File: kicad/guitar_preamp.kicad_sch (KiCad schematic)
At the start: 42 parts, among them J1 IN (от SW1B, экранир. провод), J2 BAT+ (TP4056 OUT+), J3 OUT (к SW1A) / GND, J4 Выход 6.3 Mono, J5 Звукосниматели: COM/GND, J6 TP4056 OUT+/OUT-, J7 LED (A / K), SW1 DPDT push-pull RV1, U1 MCP6022/OPA2316

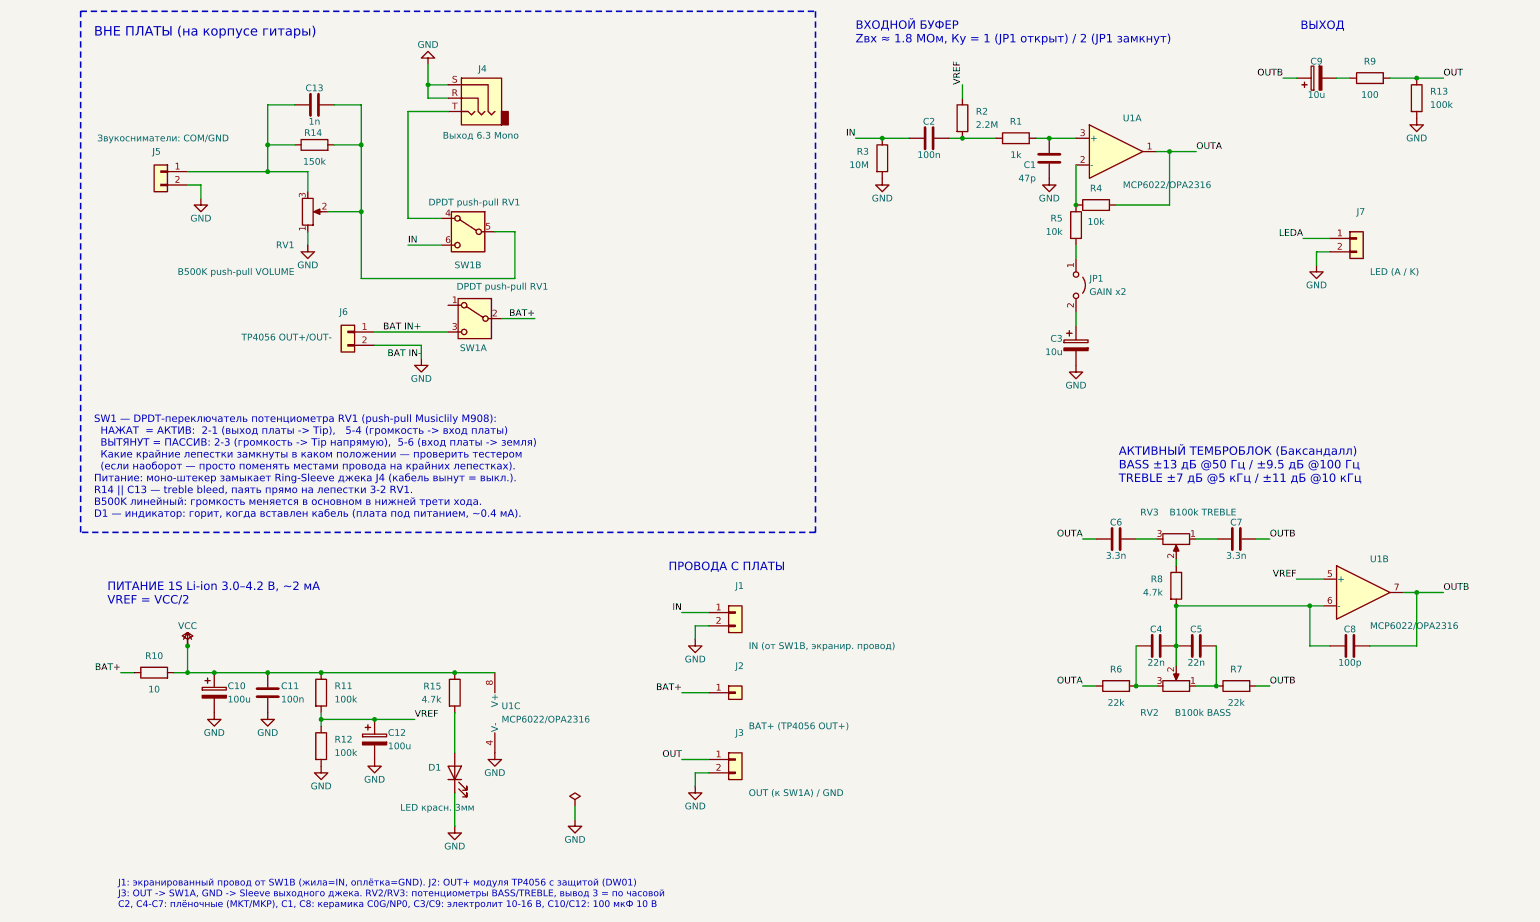
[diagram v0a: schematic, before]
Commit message: кутерьма с коннекторами
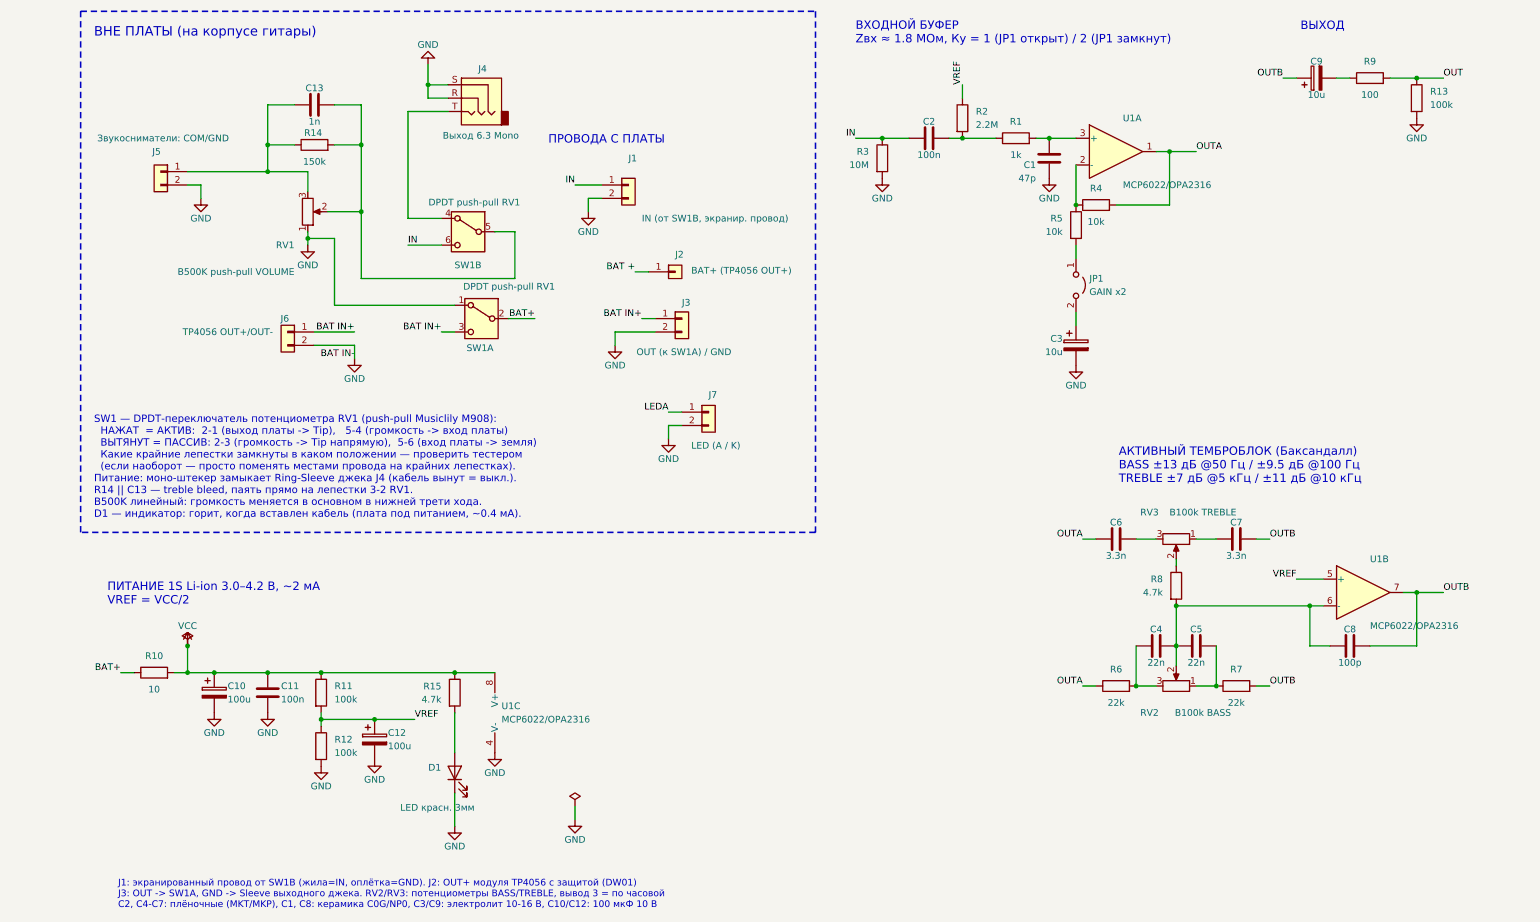
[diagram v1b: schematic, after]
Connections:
- net BAT IN+: now also J3.1 (Pin_1)
- net BAT+: no longer J2.1 (Pin_1)
- net GND: now also SW1.1 (A)
- net OUT: no longer J3.1 (Pin_1)
- new net BAT +: J2.1 (Pin_1)
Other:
- moved on the sheet: J1, J2, J3, J6, J7, SW1A
